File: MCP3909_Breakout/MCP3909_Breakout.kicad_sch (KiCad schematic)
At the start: 29 parts, among them J1 Conn_01x10, Y1 Crystal_Small

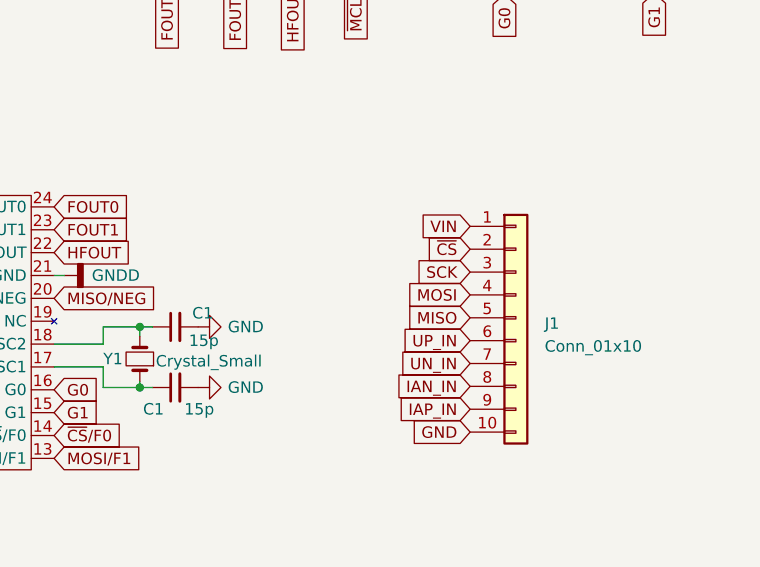
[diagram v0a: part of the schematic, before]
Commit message: First go at place-n-route
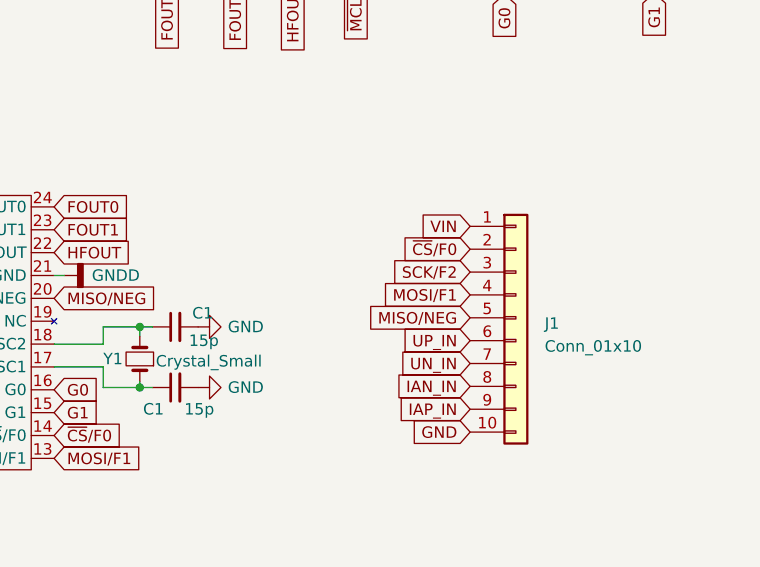
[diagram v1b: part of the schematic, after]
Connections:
- net MISO is gone; now on net MISO/NEG: J1.5 (Pin_5)
- net MOSI is gone; now on net MOSI/F1: J1.4 (Pin_4)
- net SCK is gone; now on net SCK/F2: J1.3 (Pin_3)
- net ~{CS} is gone; now on net ~{CS}/F0: J1.2 (Pin_2)
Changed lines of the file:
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@@
     )
   )
-  (global_label "MOSI" (shape input) (at 210.947 86.868 180) (fields_autoplaced)
+  (global_label "MOSI{slash}F1" (shape input) (at 210.947 86.868 180) (fields_autoplaced)
     (effects (font (size 1.27 1.27)) (justify right))
-    (property "Intersheetrefs" "${INTERSHEET_REFS}" (at 203.3656 86.868 0)
+    (property "Intersheetrefs" "${INTERSHEET_REFS}" (at 199.737 86.868 0)
       (effects (font (size 1.27 1.27)) (justify right) hide)
     )
@@
     )
   )
-  (global_label "SCK" (shape input) (at 210.947 84.328 180) (fields_autoplaced)
+  (global_label "SCK{slash}F2" (shape input) (at 210.947 84.328 180) (fields_autoplaced)
     (effects (font (size 1.27 1.27)) (justify right))
-    (property "Intersheetrefs" "${INTERSHEET_REFS}" (at 204.2917 84.328 0)
+    (property "Intersheetrefs" "${INTERSHEET_REFS}" (at 200.5837 84.328 0)
       (effects (font (size 1.27 1.27)) (justify right) hide)
     )
@@
     )
   )
-  (global_label "MISO" (shape input) (at 210.947 89.408 180) (fields_autoplaced)
+  (global_label "MISO{slash}NEG" (shape input) (at 210.947 89.408 180) (fields_autoplaced)
     (effects (font (size 1.27 1.27)) (justify right))
-    (property "Intersheetrefs" "${INTERSHEET_REFS}" (at 203.3656 89.408 0)
+    (property "Intersheetrefs" "${INTERSHEET_REFS}" (at 198.2856 89.408 0)
       (effects (font (size 1.27 1.27)) (justify right) hide)
     )
@@
     )
   )
-  (global_label "~{CS}" (shape input) (at 210.947 81.788 180) (fields_autoplaced)
+  (global_label "~{CS}{slash}F0" (shape input) (at 210.947 81.788 180) (fields_autoplaced)
     (effects (font (size 1.27 1.27)) (justify right))
-    (property "Intersheetrefs" "${INTERSHEET_REFS}" (at 205.4823 81.788 0)
+    (property "Intersheetrefs" "${INTERSHEET_REFS}" (at 201.8537 81.788 0)
       (effects (font (size 1.27 1.27)) (justify right) hide)
     )
